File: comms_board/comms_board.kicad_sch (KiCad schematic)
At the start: 0 parts

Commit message: finished placing all current components into the circuit schematic. No orginization done whatsoever
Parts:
- added C1: C_Feedthrough, CustomParts:FIL_NFM31KC103R1H3L, symbol Device:C_Feedthrough
- added C2: 27pF, Capacitor_SMD:C_1206_3216Metric_Pad1.33x1.80mm_HandSolder, symbol Device:C
- added C3: 10uF - Large Film Cap, Capacitor_THT:C_Rect_L26.5mm_W10.5mm_P22.50mm_MKS4, symbol Device:C
- added C4: 100nF - Through Hole Film Cap, Capacitor_THT:C_Axial_L17.0mm_D6.5mm_P20.00mm_Horizontal, symbol Device:C
- added D1: BAV199DW, Package_TO_SOT_SMD:SOT-363_SC-70-6, symbol Diode:BAV199DW
- added D2: BAT54S, Package_TO_SOT_SMD:SOT-23, symbol Diode:BAT54S
- added D3: Green LED, CustomParts:Untitled, symbol Device:LED
- added D4: Red LED, CustomParts:Untitled, symbol Device:LED
- added D5: Yellow LED, CustomParts:Untitled, symbol Device:LED
- added FL1: Common Mode Choke, Inductor_SMD:L_CommonMode_Wurth_WE-CNSW-1206, symbol Filter:Choke_CommonMode_FerriteCore_1243
- added J1: Molex 6 Pin Conn, Connector_Molex:Molex_Mini-Fit_Jr_5566-06A2_2x03_P4.20mm_Vertical, symbol 39299062:39299062
- added J2: 39293086, Connector_Molex:Molex_Mini-Fit_Jr_5566-08A_2x04_P4.20mm_Vertical, symbol 39293086:39293086
- added Q1: MMBT3904, Package_TO_SOT_SMD:SOT-23, symbol Transistor_BJT:MMBT3904
- added Q2: MMBT3906, Package_TO_SOT_SMD:SOT-23, symbol Transistor_BJT:MMBT3906
- added Q3: 2N7002, Package_TO_SOT_SMD:SOT-23, symbol Transistor_FET:2N7002
- added Q4: Q_Dual_NPN_NPN_E1B1C2E2B2C1, Package_TO_SOT_SMD:SOT-363_SC-70-6, symbol Transistor_BJT:Q_Dual_NPN_NPN_E1B1C2E2B2C1
- added SW1: SW_Coded_SH-7030, Button_Switch_THT:Nidec_Copal_SH-7010C, symbol Switch:SW_Coded_SH-7030
- added U1: AVR128DA48x-xPT, Package_QFP:TQFP-48_7x7mm_P0.5mm, symbol MCU_Microchip_AVR_Dx:AVR128DA48x-xPT
- added U10: REF3040 4.096 Ref Voltage, Package_TO_SOT_SMD:SOT-23, symbol Reference_Voltage:REF3040
- added U2: LTV-817S, Package_DIP:SMDIP-4_W9.53mm, symbol Isolator:LTV-817S
- added U3: INA826, Package_SO:SOIC-8_3.9x4.9mm_P1.27mm, symbol Amplifier_Instrumentation:INA821xD
- added U4: MCP25625x-x-SS, Package_SO:SSOP-28_5.3x10.2mm_P0.65mm, symbol Interface_CAN_LIN:MCP25625x-x-SS
- added U5: L7812 +12V Lin Reg, Package_TO_SOT_THT:TO-220-3_Vertical, symbol Regulator_Linear:L7812
- added U6: L7912 -12V Lin Reg, Package_TO_SOT_THT:TO-220-3_Vertical, symbol Regulator_Linear:L7912
- added U7: L7805 +5V Lin Reg, Package_TO_SOT_THT:TO-220-3_Vertical, symbol Regulator_Linear:L7805
- added U8: OPA2140, Package_SO:SOIC-8_3.9x4.9mm_P1.27mm, symbol Amplifier_Operational:OPA2134
- added U9: LM358, Package_SO:SOIC-8_3.9x4.9mm_P1.27mm, symbol Amplifier_Operational:LM358
- added Y1: 16MHz CXO, Crystal:Crystal_SMD_3225-4Pin_3.2x2.5mm, symbol Oscillator:SG-210SCD
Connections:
- new net: U1.14 (VDD), U1.42 (VDD)
- new net: U1.15 (GND), U1.29 (GND), U1.43 (GND)

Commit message: more changes to comms board
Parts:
- removed U1: AVR128DA48x-xPT, Package_QFP:TQFP-48_7x7mm_P0.5mm, symbol MCU_Microchip_AVR_Dx:AVR128DA48x-xPT
- added C10, C9: 27pF, Capacitor_SMD:C_1206_3216Metric_Pad1.33x1.80mm_HandSolder, symbol Device:C
- added C11, C12, C13, C14, C15, C16, C17, C18: 100n, Capacitor_SMD:C_1206_3216Metric_Pad1.33x1.80mm_HandSolder, symbol Device:C
- added J10: USB to UART Conn, symbol Connector:Conn_01x06_Pin
- added J3: X5, Connector_Molex:Molex_Mini-Fit_Jr_5566-08A_2x04_P4.20mm_Vertical, symbol 39293086:39293086
- added J4: X7, Connector_Molex:Molex_Mini-Fit_Jr_5566-06A2_2x03_P4.20mm_Vertical, symbol 39299062:39299062
- added J5: X9 LOCAL CAN Feedthrough Connector, Connector_Dsub:DSUB-9_Pins_Horizontal_P2.77x2.84mm_EdgePinOffset9.40mm, symbol Connector:DE9_Pins
- added J6: X8: LOCAL CAN Host Interface, Connector_Dsub:DSUB-9_Pins_Horizontal_P2.77x2.84mm_EdgePinOffset9.40mm, symbol Connector:DE9_Pins
- added J7: Pins to select 120 terminal resistance or not, TerminalBlock:TerminalBlock_MaiXu_MX126-5.0-03P_1x03_P5.00mm, symbol Connector:Conn_01x03_Pin
- added J8: UPDI Friend Input Terminal, symbol Connector:Screw_Terminal_01x03
- added R3: 120, symbol Device:R_US
- added U13: AVR128DB48x-xPT, Package_QFP:TQFP-48_7x7mm_P0.5mm, symbol MCU_Microchip_AVR_Dx:AVR128DB48x-xPT
- J1: value Molex 6 Pin Conn -> X6
- J2: value 39293086 -> X4
- SW1: value SW_Coded_SH-7030 -> DIP Switch
- U4: value MCP25625x-x-SS -> MCP25625 - CAN Transciever
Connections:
- net +15V: now reaches U7.1 (IN)
- net +15V: now also J2.6, C11.1
- net GND: now reaches U7.2 (GND)
- net GND: now also SW1.C, U4.5 (STBY), Y1.2 (GND), Y1.4 (GND), C10.1, C11.2, C12.2, C13.2, C14.2, C15.2, C16.1, C17.1, C18.2, C9.2, J10.1 (Pin_1), J5.3, J5.6, J6.3, J6.6, J8.1 (Pin_1), U13.15 (GND), U13.29 (AGND), U13.43 (GND)
- net +5V: now reaches U7.3 (OUT)
- net +5V: now also J2.2, U4.1 (V_{IO}), U4.19 (V_{DD}), U4.27 (V_{DDA}), C12.1, C13.1, C14.1, C15.1, C16.2, C17.2, C18.1, U13.14 (VDDIO2), U13.28 (AVDD), U13.42 (VDD)
- net at SW1.1: now also U13.21 (PD1)
- net at SW1.2: now also U13.22 (PD2)
- net at SW1.4: now also U13.23 (PD3)
- net at SW1.8: now also U13.24 (PD4)
- net INT: now reaches U4.13 (~{INT})
- net INT: now also U13.4 (PB0)
- net SCK: now reaches U4.14 (SCK)
- net SCK: now also U13.2 (PA6)
- net MOSI: now reaches U4.15 (SI)
- net MOSI: now also U13.48 (PA4)
- net MISO: now reaches U4.16 (SO)
- net MISO: now also U13.1 (PA5)
- net CS: now reaches U4.17 (~{CS})
- net CS: now also U13.3 (PA7)
- net RESET: now reaches U4.18 (~{RESET})
- net at U4.20 (TxCAN): now also U4.24 (T_{XD})
- net at U4.21 (RxCAN): now also U4.28 (R_{XD})
- net CAN L FILT: now reaches U4.3 (CANL)
- net CAN L FILT: now also FL1.3, J7.1 (Pin_1)
- net CAN H FILT: now reaches U4.4 (CANH)
- net CAN H FILT: now also FL1.2, R3.2
- net at U4.8 (OSC2): now also Y1.3 (OUT), C9.1
- net at U4.9 (OSC1): now also Y1.1 (IN), C10.2
- net CAN H: now reaches FL1.1
- net CAN H: now also J5.7, J6.7
- net CAN L: now reaches FL1.4
- net CAN L: now also J5.2, J6.2
- net GND1: now reaches J2.1
- net GND1: now also J2.3, J2.7
- net ACTIV HV2/: now reaches J2.4
- net ACTIV HV1/: now reaches J2.5
- net -15V: now reaches J2.8
- new net: J7.2 (Pin_2), J7.3 (Pin_3), R3.1
- new net HV1 Indicator LED Anode: J3.4
- new net HV1 Indicator LED Cathode: J3.8
- new net HV1 ON: J3.1
- new net HV1 RETURN: J3.5
- new net HV2 Indicator LED Anode: J3.3
- new net HV2 Indicator LED Cathode: J3.7
- new net HV2 ON: J3.2
- new net HV2 RETURN: J3.6
- new net RX: J10.5 (Pin_5), U13.44 (XTALHF1/PA0)
- new net TX: J10.4 (Pin_4), U13.45 (XTALHF2/PA1)
- new net UPDI Wire: J8.3 (Pin_3), U13.41 (UPDI)
- no-connect marks 0 -> 4
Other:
- added sheet Indicator Lights (Indicator Lights.kicad_sch)
- added sheet Power (Power.kicad_sch)
- note added: "Not entirely sure still how the whole board is grounded. seems to have some kind of internal ground?? Idk, definitely not just one big common GND though"
- note added: "This breakout board will be for writing code to AVR"
- note added: "Wiring to signify ID to scream into CAN. Pull down. truth table in datasheet"
- moved on the sheet: C1, C2, C3, C4, D1A, D2, D3, D4, D5, FL1, J1, J2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

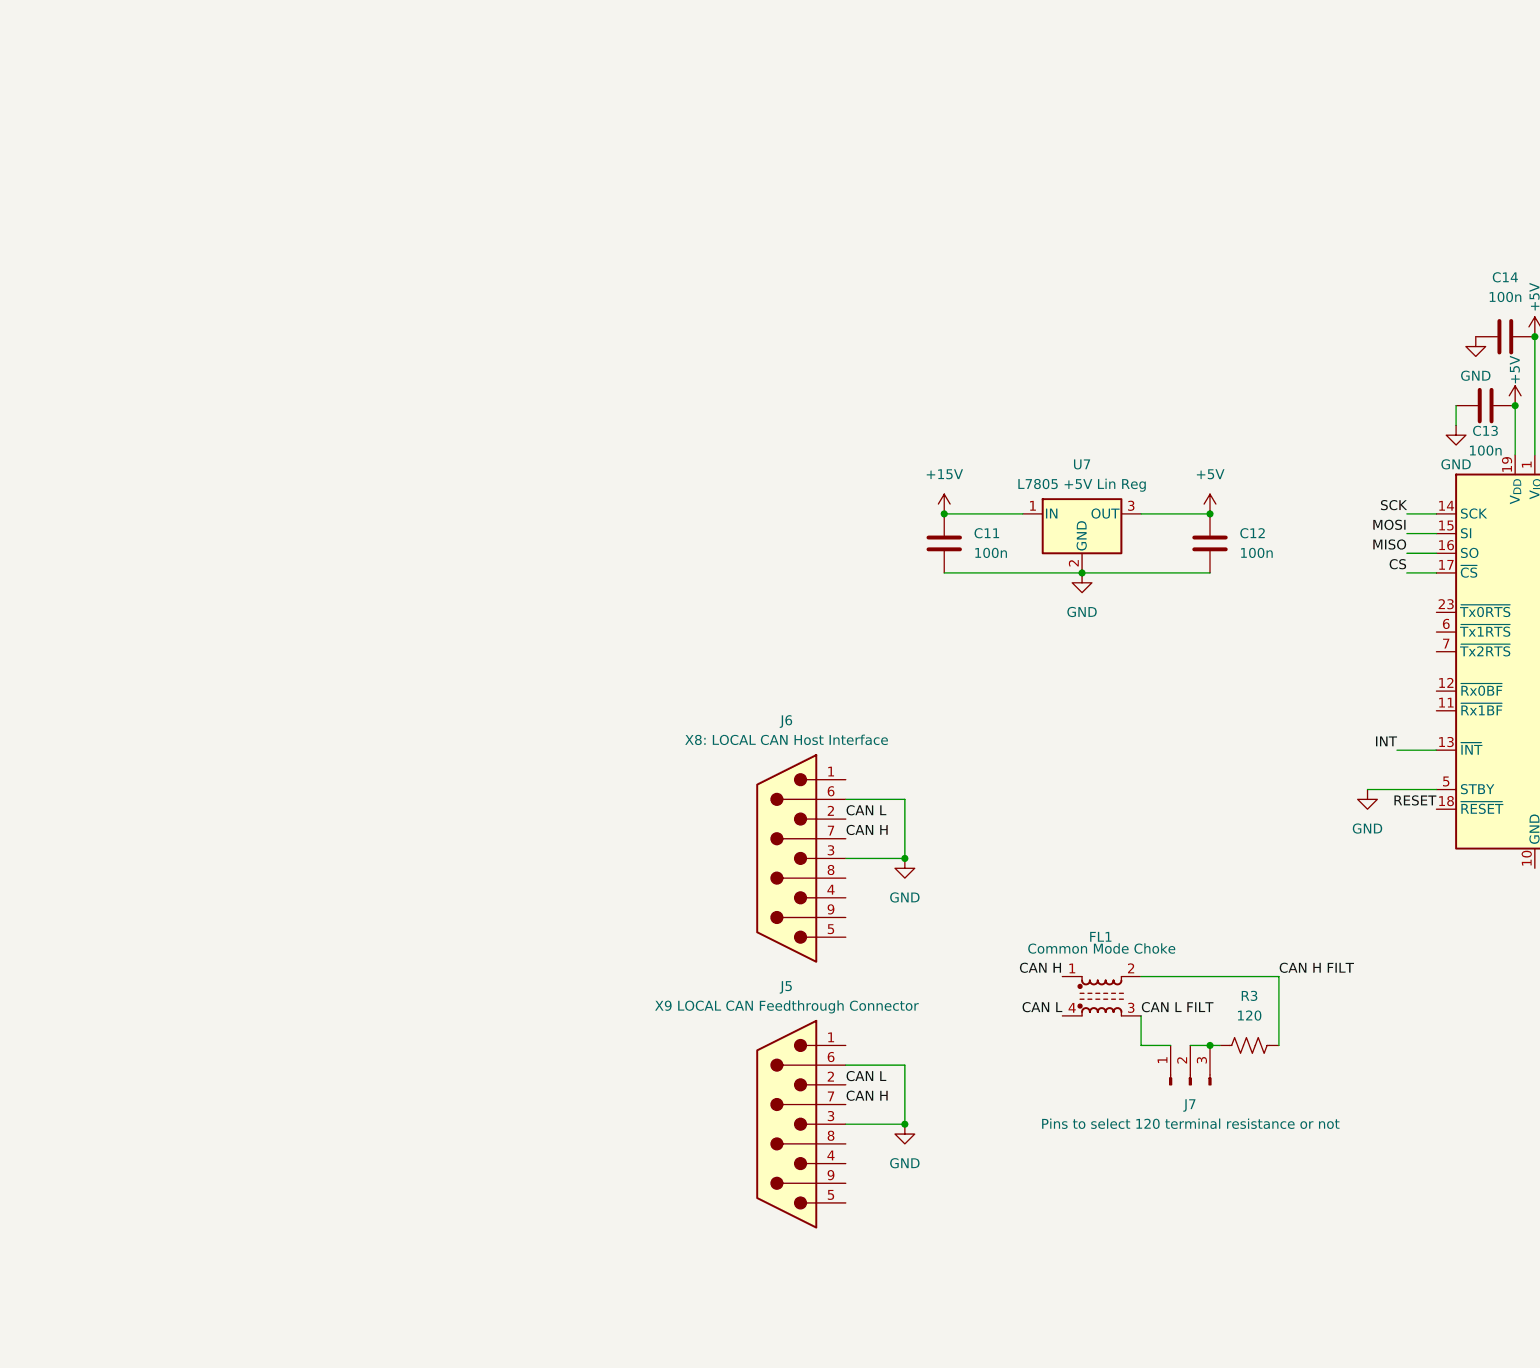
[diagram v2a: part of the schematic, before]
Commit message: finished comms test board?
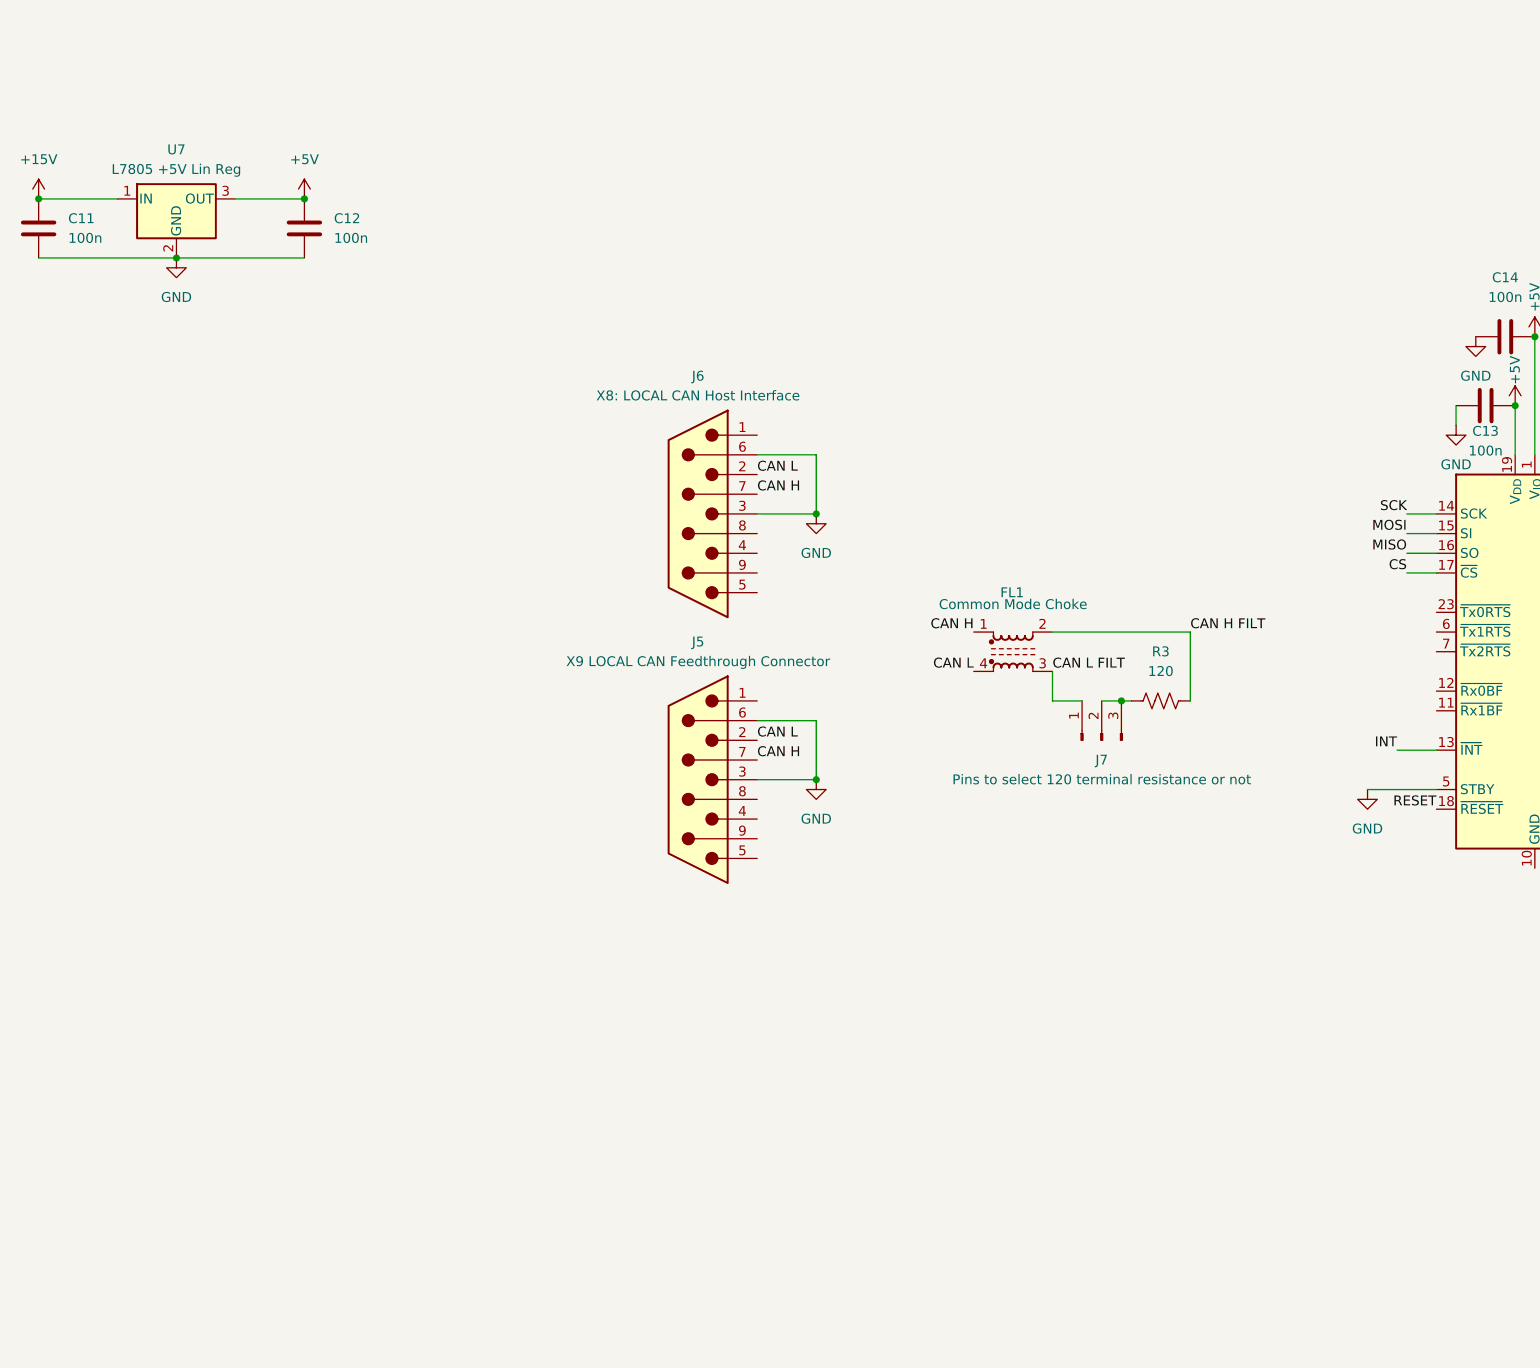
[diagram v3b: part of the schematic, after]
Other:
- moved on the sheet: C11, C12, FL1, J5, J6, J7, R3, U7
